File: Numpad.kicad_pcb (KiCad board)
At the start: 2 copper layers, 88.9 x 104.8 mm, 50 parts, among them SW1 SW_Push, U1 ATmega32U4-AU, Y1 16MHz

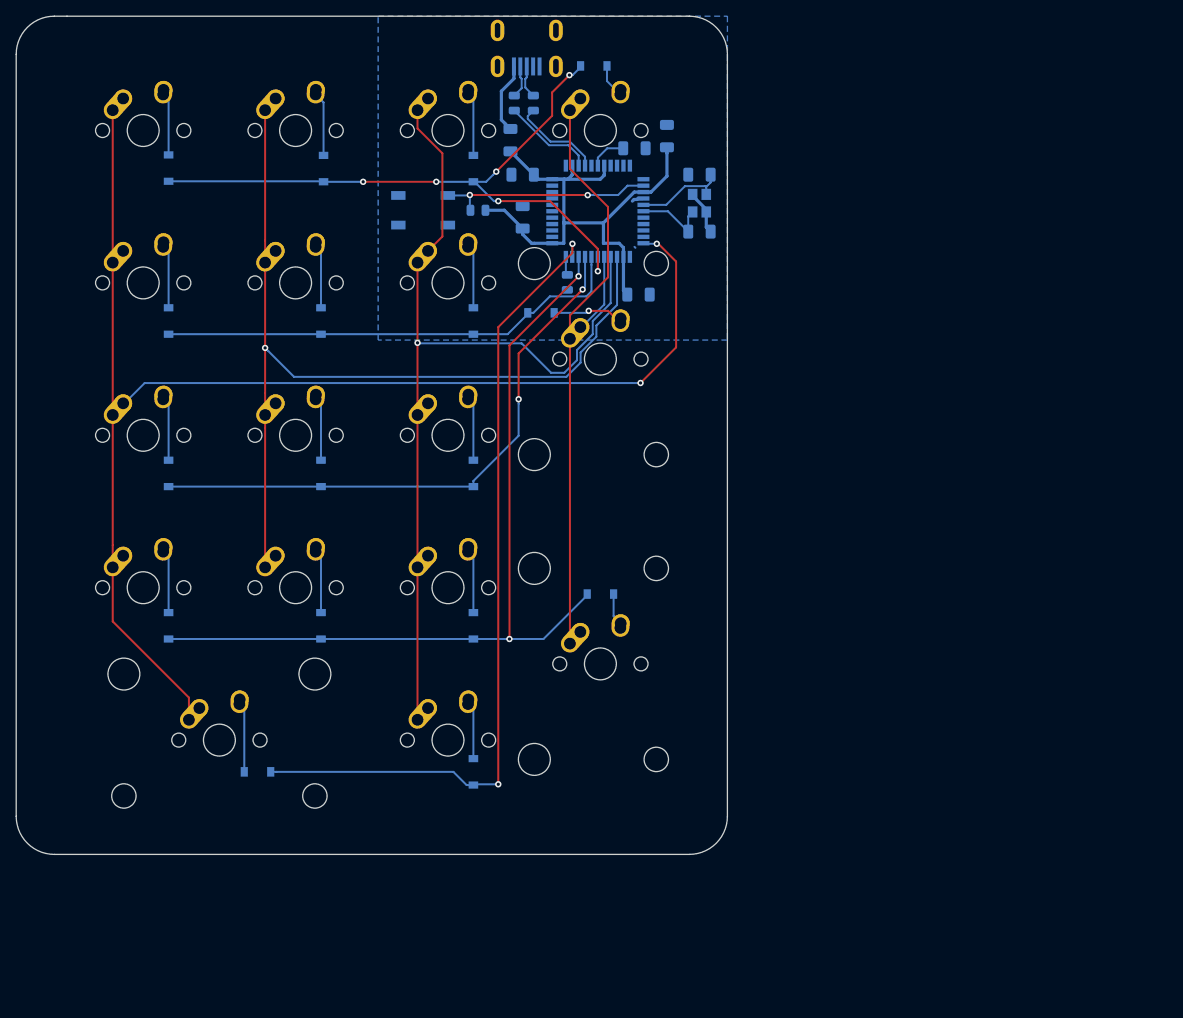
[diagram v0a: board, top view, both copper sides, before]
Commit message: Restart project
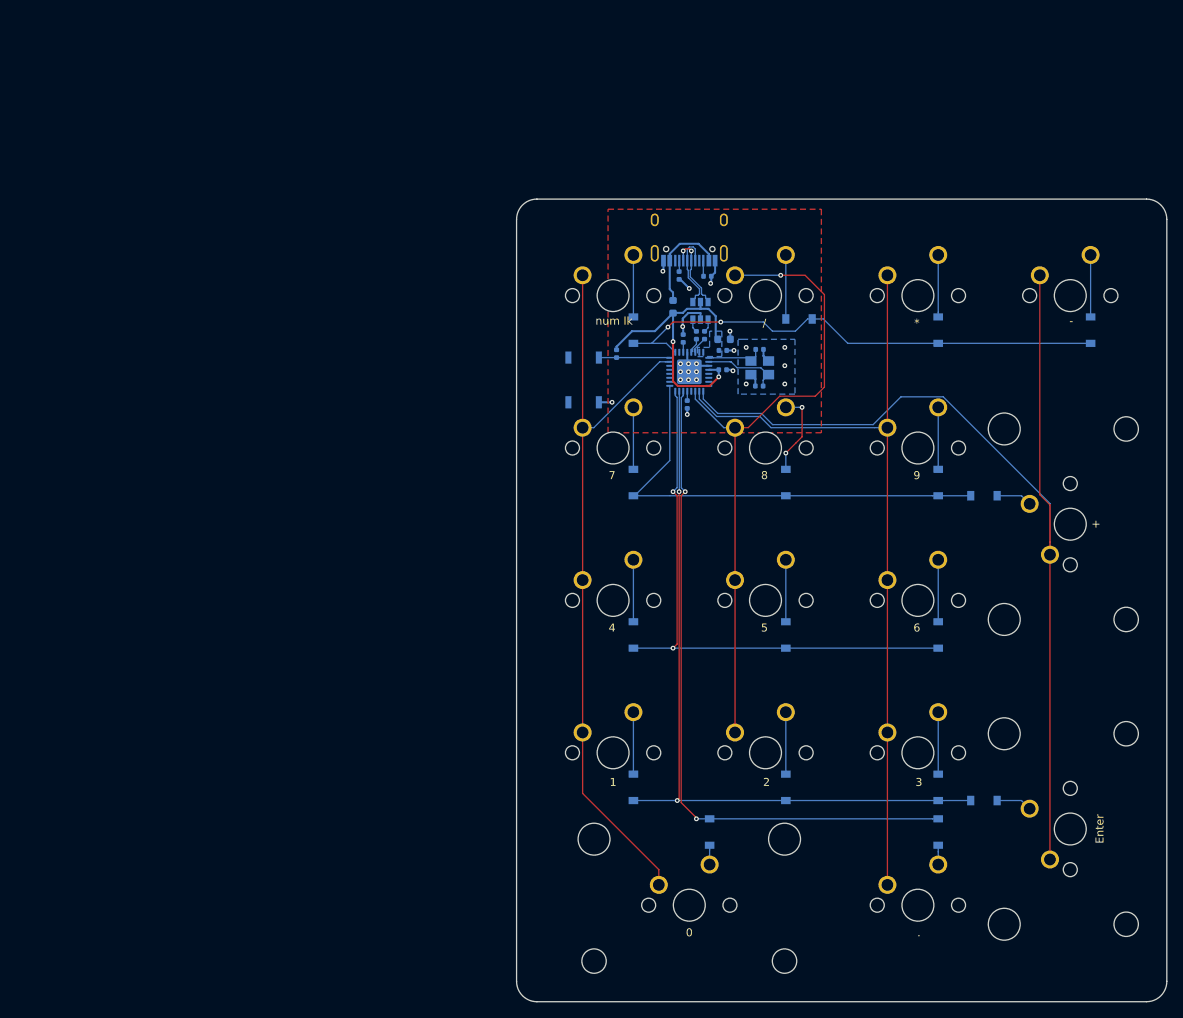
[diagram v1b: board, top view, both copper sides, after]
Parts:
- removed C7: 1uF, Capacitor_SMD:C_1206_3216Metric
- removed D14, D15, D16, D17, D4, D5, D6, D7, D8, D9: D_Small, Diode_SMD:D_SOD-123
- removed MX14, MX17, MX4, MX5, MX6, MX7, MX9: MX-NoLED, MX_Alps_Hybrid:MX-1U-NoLED
- removed MX15, MX8: MX-NoLED, MX_Alps_Hybrid:MX-2U-ReversedStabilizers-Vertical-NoLED
- removed MX16: MX-NoLED, MX_Alps_Hybrid:MX-2U-ReversedStabilizers-NoLED
- added D0: D_Small_ALT, Diode_SMD:D_SOD-123, B.Cu at (94.6, 58.3)
- added D20: D_Small_ALT, Diode_SMD:D_SOD-123, B.Cu at (94.6, 96.4)
- added D21: D_Small_ALT, Diode_SMD:D_SOD-123, B.Cu at (113.7, 96.4)
- added D22: D_Small_ALT, Diode_SMD:D_SOD-123, B.Cu at (132.7, 96.4)
- added D30: D_Small_ALT, Diode_SMD:D_SOD-123, B.Cu at (94.6, 115.4)
- added D31: D_Small_ALT, Diode_SMD:D_SOD-123, B.Cu at (113.7, 115.4)
- added D32: D_Small_ALT, Diode_SMD:D_SOD-123, B.Cu at (132.7, 115.4)
- added D33: D_Small_ALT, Diode_SMD:D_SOD-123, B.Cu at (138.4, 117.1)
- added D40: D_Small_ALT, Diode_SMD:D_SOD-123, B.Cu at (104.1, 121.0)
- added D42: D_Small_ALT, Diode_SMD:D_SOD-123, B.Cu at (132.7, 121.0)
- added MX0: MX-NoLED, MX_Only:MXOnly-1U-NoLED, F.Cu at (92.1, 54.0)
- added MX20: MX-NoLED, MX_Only:MXOnly-1U-NoLED, F.Cu at (92.1, 92.1)
- added MX21: MX-NoLED, MX_Only:MXOnly-1U-NoLED, F.Cu at (111.1, 92.1)
- added MX22: MX-NoLED, MX_Only:MXOnly-1U-NoLED, F.Cu at (130.2, 92.1)
- added MX30: MX-NoLED, MX_Only:MXOnly-1U-NoLED, F.Cu at (92.1, 111.1)
- added MX31: MX-NoLED, MX_Only:MXOnly-1U-NoLED, F.Cu at (111.1, 111.1)
- added MX32: MX-NoLED, MX_Only:MXOnly-1U-NoLED, F.Cu at (130.2, 111.1)
- added MX33: MX-NoLED, MX_Only:MXOnly-2U-ReversedStabilizers-NoLED, F.Cu at (149.2, 120.7)
- added MX40: MX-NoLED, MX_Only:MXOnly-2U-ReversedStabilizers-NoLED, F.Cu at (101.6, 130.2)
- added MX42: MX-NoLED, MX_Only:MXOnly-1U-NoLED, F.Cu at (130.2, 130.2)
- added R5: 22R, Resistor_SMD:R_0402_1005Metric, B.Cu at (103.5, 58.9)
- added R6: 10k, Resistor_SMD:R_0402_1005Metric, B.Cu at (101.3, 67.6)
- added U2: ATmega32U2-MU, Package_DFN_QFN:QFN-32-1EP_5x5mm_P0.5mm_EP3.1x3.1mm, B.Cu at (101.6, 63.5)
- C1, C2: value 22pF -> 100nF; footprint Capacitor_SMD:C_1206_3216Metric -> Capacitor_SMD:C_0402_1005Metric
- C3: value 0.1uF -> 10uF; footprint Capacitor_SMD:C_1206_3216Metric -> Capacitor_SMD:C_0603_1608Metric
- C4, C5: value 0.1uF -> 22pF; footprint Capacitor_SMD:C_1206_3216Metric -> Capacitor_SMD:C_0402_1005Metric
- C6: value 10uF -> 1uF; footprint Capacitor_SMD:C_1206_3216Metric -> Capacitor_SMD:C_0402_1005Metric
- D1, D10, D11, D12, D13, D2, D3: value D_Small -> D_Small_ALT
- F1: footprint Fuse:Fuse_1206_3216Metric -> Fuse:Fuse_0603_1608Metric
- MX1, MX10, MX11, MX12, MX2, MX3: footprint MX_Alps_Hybrid:MX-1U-NoLED -> MX_Only:MXOnly-1U-NoLED
- MX13: footprint MX_Alps_Hybrid:MX-1U-NoLED -> MX_Only:MXOnly-2U-ReversedStabilizers-NoLED
- R1: value 10k -> 5.1k; footprint Resistor_SMD:R_0805_2012Metric -> Resistor_SMD:R_0402_1005Metric
- R2: value 22 -> 5.1k; footprint Resistor_SMD:R_0805_2012Metric -> Resistor_SMD:R_0402_1005Metric
- R3: value 22 -> 10k; footprint Resistor_SMD:R_0805_2012Metric -> Resistor_SMD:R_0402_1005Metric
- R4: value 10k -> 22R; footprint Resistor_SMD:R_0805_2012Metric -> Resistor_SMD:R_0402_1005Metric
- SW1: footprint random-keyboard-parts:SKQG-1155865 -> Switches:TACTILE_SWITCH_SMD_5.2MM
- U1: value ATmega32U4-AU -> USBLC6-2SC6; footprint Package_QFP:TQFP-44_10x10mm_P0.8mm -> Package_TO_SOT_SMD:SOT-23-6
- USB1: value Molex-0548190589 -> HRO-TYPE-C-31-M-12; footprint random-keyboard-parts:Molex-0548190589 -> Type-C:HRO-TYPE-C-31-M-12
- moved MX12 98.4 mm to (130.2, 73.0)
- moved D12 97.9 mm to (132.7, 77.3)
- moved MX13 97.2 mm to (149.2, 82.5), turned to 90 degrees
- moved D13 84.4 mm to (138.4, 79.0), turned to 0 degrees
- moved D1 81.0 mm to (115.3, 56.9), turned to 180 degrees
- moved MX2 80.5 mm to (130.2, 54.0)
- moved MX1 80.5 mm to (111.1, 54.0)
- moved MX3 80.5 mm to (149.2, 54.0)
- moved D3 79.8 mm to (151.8, 58.3)
- moved D2 79.4 mm to (132.7, 58.3)
- moved MX10 39.7 mm to (92.1, 73.0)
- moved MX11 39.7 mm to (111.1, 73.0)
- moved C5 39.6 mm to (110.3, 65.3)
- moved D11 39.1 mm to (113.7, 77.3)
- moved D10 39.1 mm to (94.6, 77.3)
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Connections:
- C1 pad 1: GND -> +5V
- C1 pad 2: Net-(C1-Pad2) -> GND
- C2 pad 1: Net-(C2-Pad1) -> +5V
- C4 pad 1: +5V -> Net-(C4-Pad1)
- C5 pad 1: +5V -> Net-(C5-Pad1)
- C6 pad 1: +5V -> Net-(C6-Pad1)
- D10 pad 1: ROW2 -> ROW1
- D11 pad 1: ROW2 -> ROW1
- D12 pad 1: ROW3 -> ROW1
- D13 pad 1: ROW3 -> ROW1
- MX1 pad 1: COL0 -> COL1
- MX10 pad 1: COL1 -> COL0
- MX11 pad 1: COL2 -> COL1
- MX12 pad 1: COL0 -> COL2
- MX13 pad 1: COL1 -> COL3
- MX2 pad 1: COL1 -> COL2
- MX3 pad 1: COL2 -> COL3
- R1 pad 1: +5V -> Net-(R1-Pad1)
- R1 pad 2: Net-(R1-Pad2) -> GND
- R2 pad 1: /USB_D+ -> Net-(R2-Pad1)
- R2 pad 2: D+ -> GND
- R3 pad 1: /USB_D- -> +5V
- R3 pad 2: D- -> Net-(R3-Pad2)
- R4 pad 1: GND -> /MCU_D+
- R4 pad 2: Net-(R4-Pad2) -> D+
- SW1 pad 2: Net-(R1-Pad2) -> Net-(R3-Pad2)
- U1 pad 1: Net-(U1-Pad1) -> D-
- U1 pad 2: +5V -> GND
- U1 pad 3: /USB_D- -> D+
- U1 pad 4: /USB_D+ -> USB_D+
- U1 pad 5: GND -> +5V
- U1 pad 6: Net-(C7-Pad1) -> USB_D-
- USB1 pad 2: Net-(USB1-Pad2) -> VCC
- USB1 pad 3: D+ -> Net-(USB1-Pad3)
- USB1 pad 4: D- -> Net-(R2-Pad1)
- USB1 pad 5: VCC -> USB_D-
- USB1 pad 6: Net-(USB1-Pad6) -> USB_D+
- Y1 pad 1: Net-(C2-Pad1) -> Net-(C4-Pad1)
- Y1 pad 3: Net-(C1-Pad2) -> Net-(C5-Pad1)
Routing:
- net COL0: track 169.8 -> 94.5 mm, vias 2 -> 0
- net COL3: track 82.6 -> 132.5 mm
- net +5V: track 68.7 -> 35.7 mm, vias 0 -> 2
- net COL1: track 114.5 -> 82.5 mm
- net Net-(R1-Pad2): track 26.9 -> 0.00 mm, vias 2 -> 0
- net GND: track 7.21 -> 26.0 mm, vias 0 -> 23
- net ROW0: track 82.8 -> 64.0 mm, vias 6 -> 2
- net ROW4: track 102.2 -> 85.0 mm
- net COL2: track 115.8 -> 102.2 mm, vias 1 -> 0
- net ROW3: track 106.1 -> 93.4 mm
- net /USB_D-: track 11.6 -> 0.00 mm
- net Net-(C2-Pad1): track 11.6 -> 0.00 mm
- net /USB_D+: track 11.6 -> 0.00 mm
- net USB_D+: track 0.00 -> 10.4 mm
- net USB_D-: track 0.00 -> 9.97 mm, vias 0 -> 2
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- added copper zone on B.Cu, net +5V
- added copper zone on F.Cu, net GND
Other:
- board size 88.9 x 104.8 mm -> 81.3 x 100.3 mm
- net class Default: clearance 0.2 -> 0.127; trace_width 0.25 -> 0.127; via_dia 0.8 -> 0.6; via_drill 0.4 -> 0.3
- net class Power: clearance 0.2 -> 0.127; trace_width 0.4 -> 0.254; via_dia 0.8 -> 0.6; via_drill 0.4 -> 0.3
- rule trace_clearance: 0.2 -> 0.127
- rule trace_min: 0.2 -> 0.127
- rule via_min_size: 0.4 -> 0.2
- board text added: "*"
- board text added: "+"
- board text added: "-"
- board text added: "."
- board text added: "/"
- board text added: "0"
- board text added: "1"
- board text added: "2"
- board text added: "3"
- board text added: "4"
- board text added: "5"
- board text added: "6"
- board text added: "7"
- board text added: "8"
- board text added: "9"
- board text added: "Enter"
- board text added: "Numpad v1 Designed by Aaron Lucas and Oliver Martin"
- board text added: "num lk"
